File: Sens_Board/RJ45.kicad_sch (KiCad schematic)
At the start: 1 part

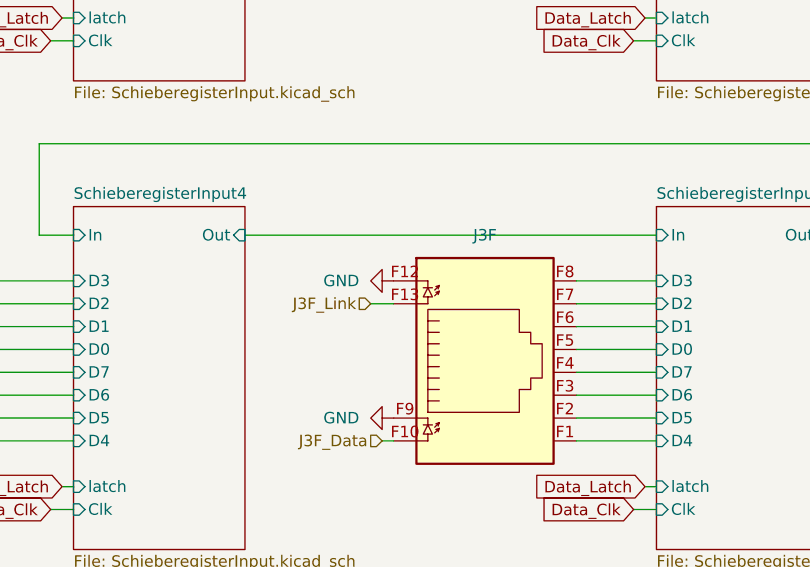
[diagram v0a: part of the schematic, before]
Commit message: Production File generate
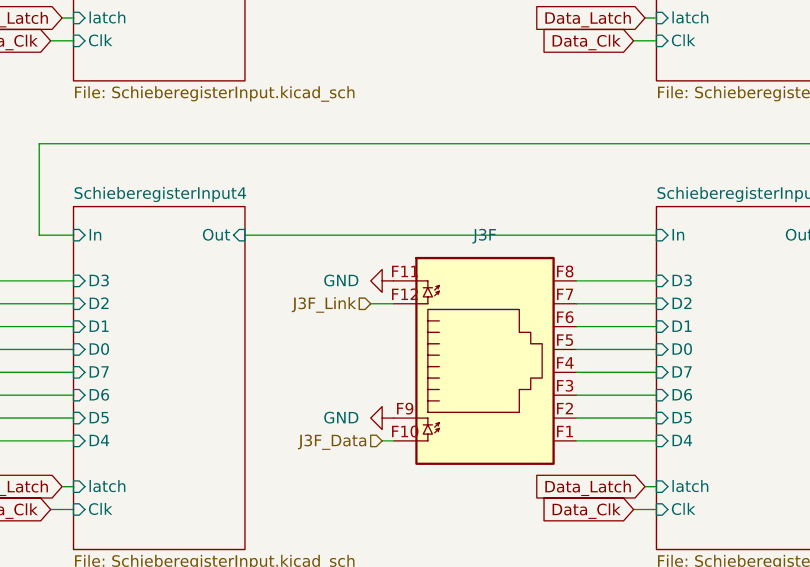
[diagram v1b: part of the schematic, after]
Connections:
- net GND: now also J3.F11; no longer J3.F12
- net J3F_Link: now also J3.F12; no longer J3.F13
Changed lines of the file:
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@@
 	)
 	(symbol
+		(lib_name "RJ45-12_1")
 		(lib_id "Techbeard:RJ45-12")
 		(at 100.33 86.36 0)
@@
 		(pin "B7"
 		)
-		(pin "F13"
+		(pin "F11"
 		)
 		(pin "E12"
